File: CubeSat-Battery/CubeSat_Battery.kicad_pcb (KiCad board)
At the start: 2 copper layers, 92 x 92 mm, 5 parts, among them J1 Conn_01x02_Pin, J2 Conn_01x02_Pin, U1 BatteryPack

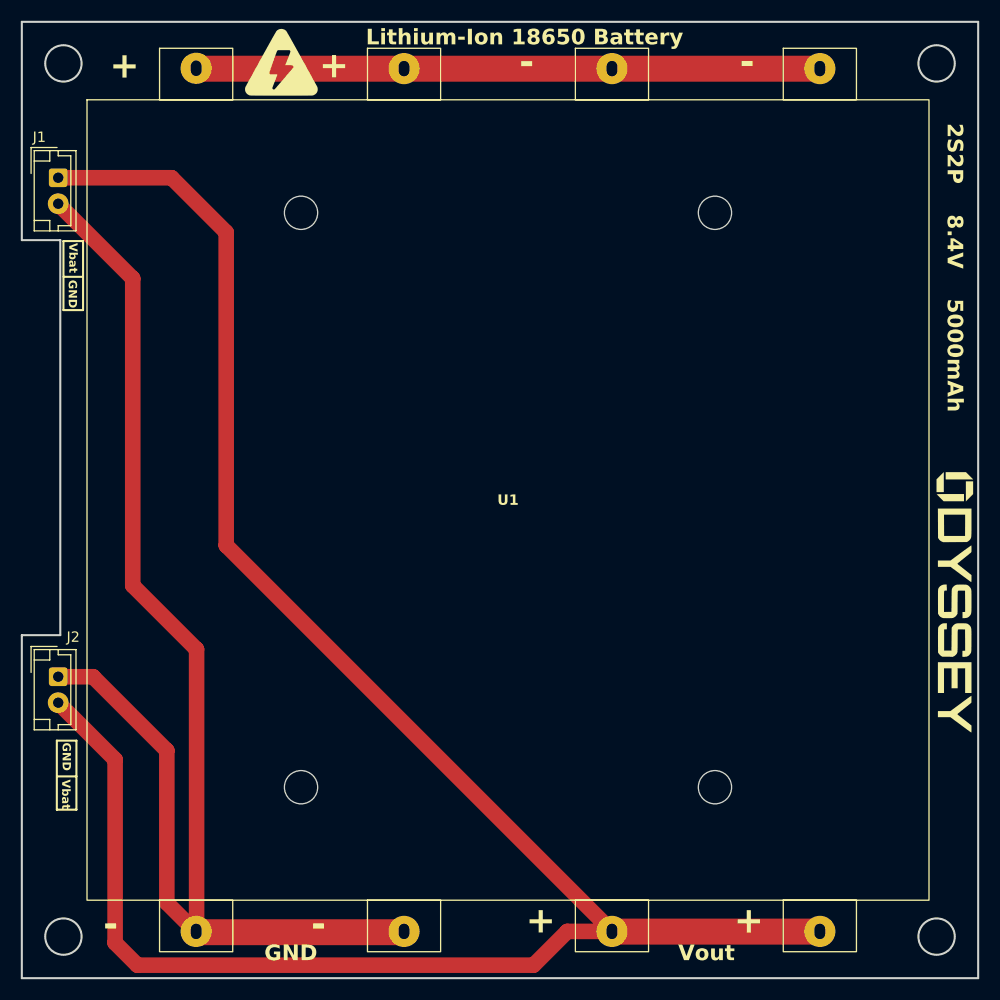
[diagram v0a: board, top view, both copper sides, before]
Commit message: final changes
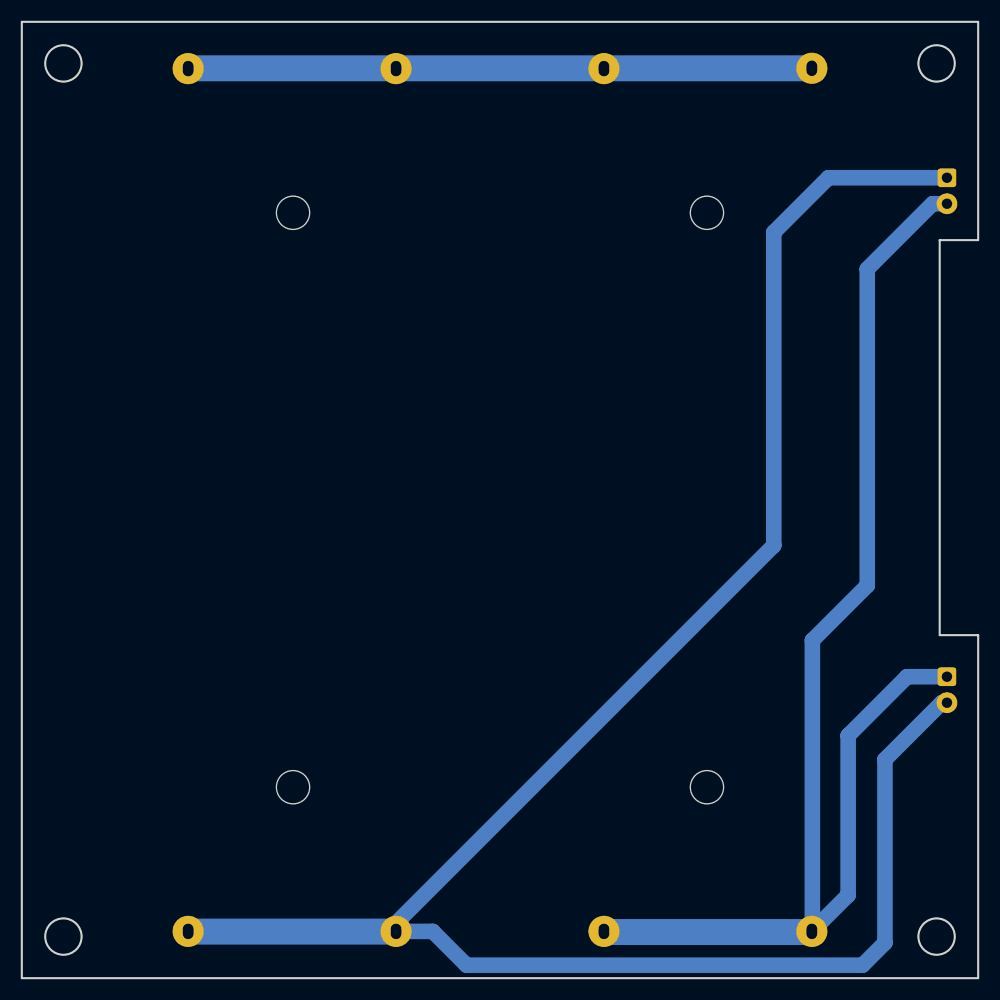
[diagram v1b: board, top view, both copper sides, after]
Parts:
- G*** (x2), J1, J2, U1: moved to B.Cu
- moved G*** 87.5 mm to (2.25, 55.9)
- moved J1 85.5 mm to (89.0, 15.0)
- moved J2 85.5 mm to (89.0, 63.0)
- moved G*** 42.1 mm to (67.0, 3.89), turned to 180 degrees
- moved U1 0.77 mm to (46.0, 46.0), turned to 180 degrees
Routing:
- net GND: track 127.4 -> 128.1 mm
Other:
- outline, holes or cut-outs redrawn
